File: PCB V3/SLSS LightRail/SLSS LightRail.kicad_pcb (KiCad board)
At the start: 2 copper layers, 18.1 x 32.8 mm, 1 part

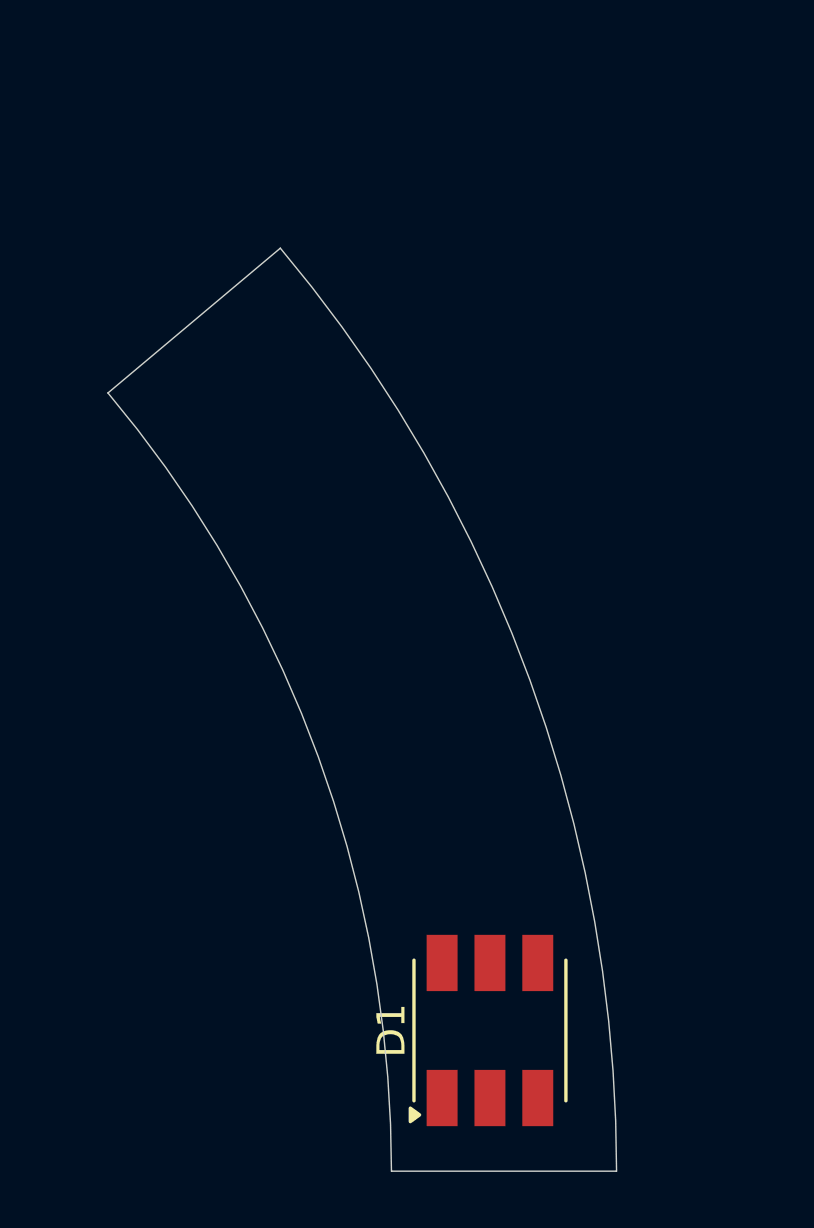
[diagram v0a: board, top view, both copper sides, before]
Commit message: light rail PCB
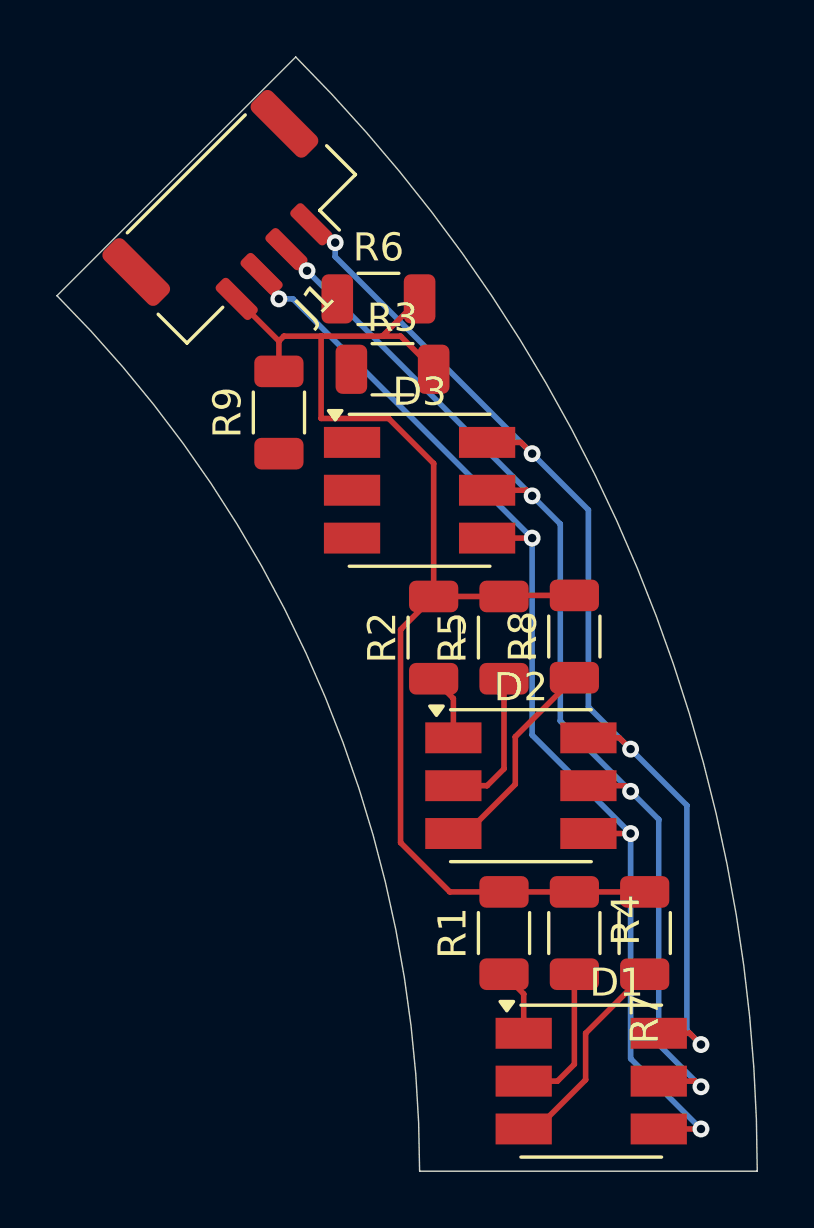
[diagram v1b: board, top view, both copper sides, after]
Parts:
- added D2: LED_RGB, LED_SMD:LED_RGB_5050-6, F.Cu at (197.6, 86.3)
- added D3: LED_RGB, LED_SMD:LED_RGB_5050-6, F.Cu at (194.0, 75.8)
- added J1: Conn_01x04, Connector_JST:JST_GH_SM04B-GHS-TB_1x04-1MP_P1.25mm_Horizontal, F.Cu at (187.5, 66.4)
- added R1: 51R, Resistor_SMD:R_1206_3216Metric, F.Cu at (197.0, 91.5)
- added R2: 51R, Resistor_SMD:R_1206_3216Metric, F.Cu at (194.5, 81.0)
- added R3: 51R, Resistor_SMD:R_1206_3216Metric, F.Cu at (193.0, 71.5)
- added R4: 62R, Resistor_SMD:R_1206_3216Metric, F.Cu at (199.5, 91.5)
- added R5: 62R, Resistor_SMD:R_1206_3216Metric, F.Cu at (197.0, 81.0)
- added R6: 62R, Resistor_SMD:R_1206_3216Metric, F.Cu at (192.5, 69.0)
- added R7: 51R, Resistor_SMD:R_1206_3216Metric, F.Cu at (202.0, 91.5)
- added R8: 51R, Resistor_SMD:R_1206_3216Metric, F.Cu at (199.5, 81.0)
- added R9: 51R, Resistor_SMD:R_1206_3216Metric, F.Cu at (189.0, 73.0)
- moved D1 4.02 mm to (200.1, 96.8), turned to 0 degrees
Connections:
- D1 pad 1: unconnected-(D1-RK-Pad1) -> Net-(D1-RK)
- D1 pad 2: unconnected-(D1-GK-Pad2) -> Net-(D1-GK)
- D1 pad 3: unconnected-(D1-BK-Pad3) -> Net-(D1-BK)
- D1 pad 4: unconnected-(D1-BA-Pad4) -> Net-(D1-BA)
- D1 pad 5: unconnected-(D1-GA-Pad5) -> Net-(D1-GA)
- D1 pad 6: unconnected-(D1-RA-Pad6) -> Net-(D1-RA)
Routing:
- net Net-(J1-Pin_4): track 0.00 -> 47.2 mm
- net Net-(D1-BA): track 0.00 -> 41.7 mm, vias 0 -> 4
- net Net-(D1-GA): track 0.00 -> 41.0 mm, vias 0 -> 4
- net Net-(D1-RA): track 0.00 -> 39.9 mm, vias 0 -> 4
- net Net-(D2-BK): track 0.00 -> 7.58 mm
- net Net-(D1-BK): track 0.00 -> 7.55 mm
- net Net-(D2-GK): track 0.00 -> 5.25 mm
- net Net-(D1-GK): track 0.00 -> 5.25 mm
- net Net-(D2-RK): track 0.00 -> 2.39 mm
- net Net-(D1-RK): track 0.00 -> 2.39 mm
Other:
- board size 18.1 x 32.8 mm -> 24.9 x 39.6 mm
- board text added: "${REFERENCE}"

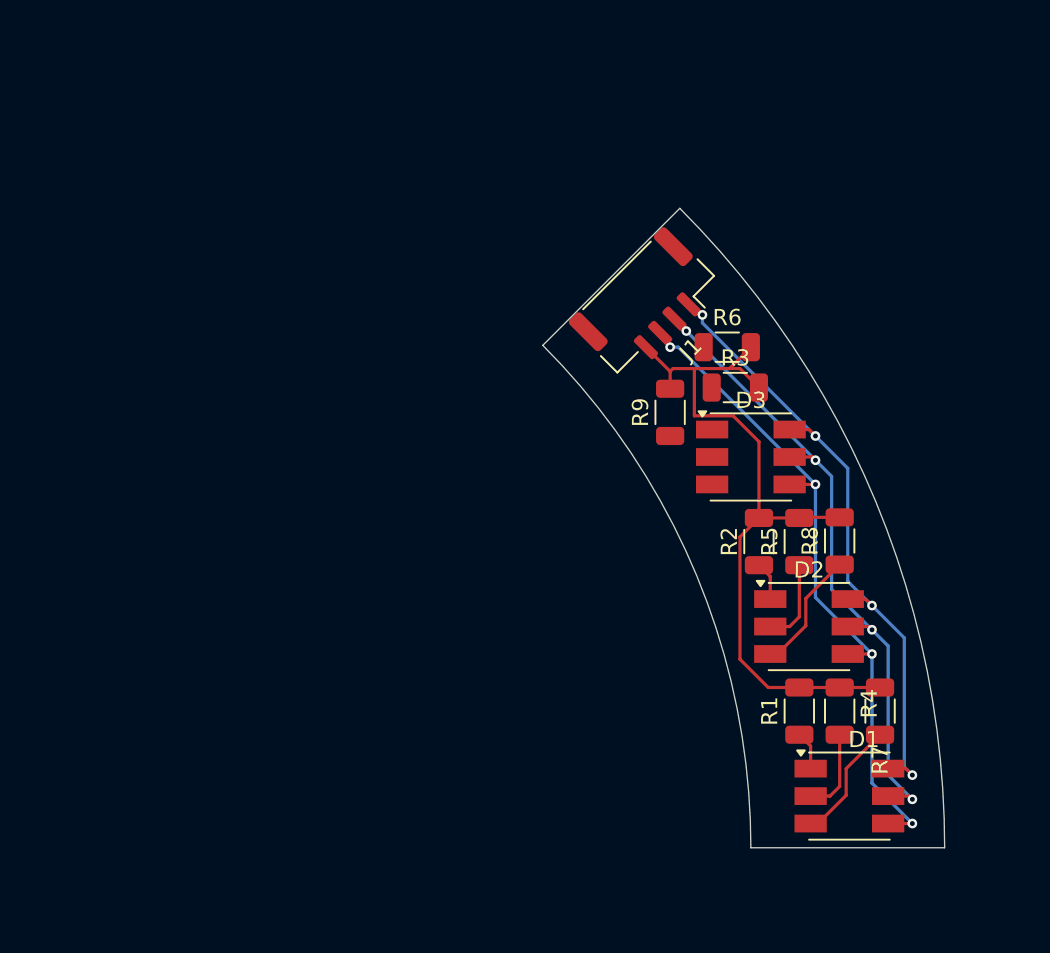
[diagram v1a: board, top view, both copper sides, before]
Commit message: Finished Lightrail PCB
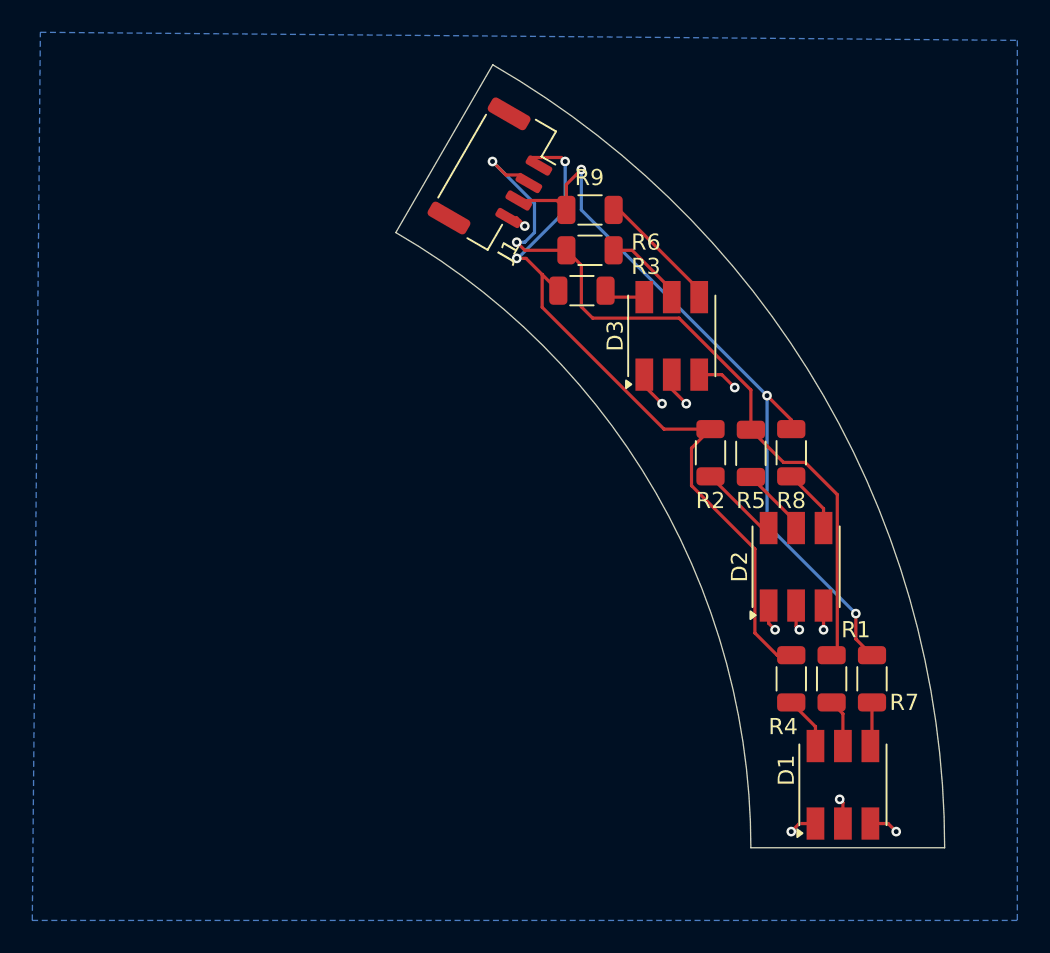
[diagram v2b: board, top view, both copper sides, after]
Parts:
- moved R9 13.5 mm to (184.0, 60.5), turned to 0 degrees
- moved J1 12.1 mm to (178.3, 58.5), turned to -120 degrees
- moved R3 11.2 mm to (183.5, 65.5)
- moved R6 10.4 mm to (184.0, 63.0)
- moved D3 8.96 mm to (189.1, 68.3), turned to 90 degrees
- moved R2 6.26 mm to (191.5, 75.5), turned to -90 degrees
- moved R8 6.23 mm to (196.5, 75.5), turned to -90 degrees
- moved R5 6.23 mm to (194.0, 75.6), turned to -90 degrees
- moved D2 3.79 mm to (196.8, 82.6), turned to 90 degrees
- moved R1 2.06 mm to (196.5, 89.5), turned to -90 degrees
- moved R4 2.06 mm to (199.0, 89.5), turned to 90 degrees
- moved R7 2.06 mm to (201.5, 89.5), turned to -90 degrees
- moved D1 0.81 mm to (199.7, 96.1), turned to 90 degrees
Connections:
- D1 pad 1: Net-(D1-RK) -> Net-(D1-BK)
- D1 pad 2: Net-(D1-GK) -> Net-(D1-BK)
- D2 pad 1: Net-(D2-RK) -> Net-(D1-BK)
- D2 pad 2: Net-(D2-GK) -> Net-(D1-BK)
- D2 pad 3: Net-(D2-BK) -> Net-(D1-BK)
- D2 pad 4: Net-(D1-BA) -> Net-(D2-BA)
- D2 pad 5: Net-(D1-GA) -> Net-(D2-GA)
- D2 pad 6: Net-(D1-RA) -> Net-(D2-RA)
- D3 pad 1: Net-(D3-RK) -> Net-(D1-BK)
- D3 pad 2: Net-(D3-GK) -> Net-(D1-BK)
- D3 pad 3: Net-(D3-BK) -> Net-(D1-BK)
- D3 pad 4: Net-(D1-BA) -> Net-(D3-BA)
- D3 pad 5: Net-(D1-GA) -> Net-(D3-GA)
- D3 pad 6: Net-(D1-RA) -> Net-(D3-RA)
- J1 pad 1: Net-(D1-RA) -> Net-(J1-Pin_1)
- J1 pad 2: Net-(D1-GA) -> Net-(J1-Pin_2)
- J1 pad 3: Net-(D1-BA) -> Net-(J1-Pin_3)
- J1 pad 4: Net-(J1-Pin_4) -> Net-(D1-BK)
- R1 pad 1: Net-(D1-RK) -> Net-(J1-Pin_1)
- R1 pad 2: Net-(J1-Pin_4) -> Net-(D1-RA)
- R2 pad 1: Net-(D2-RK) -> Net-(J1-Pin_1)
- R2 pad 2: Net-(J1-Pin_4) -> Net-(D2-RA)
- R3 pad 1: Net-(D3-RK) -> Net-(J1-Pin_1)
- R3 pad 2: Net-(J1-Pin_4) -> Net-(D3-RA)
- R4 pad 1: Net-(J1-Pin_4) -> Net-(D1-GA)
- R4 pad 2: Net-(D1-GK) -> Net-(J1-Pin_2)
- R5 pad 1: Net-(D2-GK) -> Net-(J1-Pin_2)
- R5 pad 2: Net-(J1-Pin_4) -> Net-(D2-GA)
- R6 pad 1: Net-(D3-GK) -> Net-(J1-Pin_2)
- R6 pad 2: Net-(J1-Pin_4) -> Net-(D3-GA)
- R7 pad 1: Net-(D1-BK) -> Net-(J1-Pin_3)
- R7 pad 2: Net-(J1-Pin_4) -> Net-(D1-BA)
- R8 pad 1: Net-(D2-BK) -> Net-(J1-Pin_3)
- R8 pad 2: Net-(J1-Pin_4) -> Net-(D2-BA)
- R9 pad 1: Net-(D3-BK) -> Net-(J1-Pin_3)
- R9 pad 2: Net-(J1-Pin_4) -> Net-(D3-BA)
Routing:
- net Net-(J1-Pin_2): track 0.00 -> 48.3 mm, vias 0 -> 2
- net Net-(J1-Pin_4): track 47.2 -> 0.00 mm
- net Net-(J1-Pin_3): track 0.00 -> 46.3 mm, vias 0 -> 3
- net Net-(J1-Pin_1): track 0.00 -> 46.0 mm, vias 0 -> 2
- net Net-(D1-BA): track 41.7 -> 2.74 mm, vias 4 -> 0
- net Net-(D1-GA): track 41.0 -> 2.99 mm, vias 4 -> 0
- net Net-(D1-RA): track 39.9 -> 3.32 mm, vias 4 -> 0
- net Net-(D1-BK): track 7.55 -> 18.0 mm, vias 0 -> 10
- net Net-(D3-BA): track 0.00 -> 7.80 mm
- net Net-(D2-BK): track 7.58 -> 0.00 mm
- net Net-(D2-GK): track 5.25 -> 0.00 mm
- net Net-(D1-GK): track 5.25 -> 0.00 mm
- net Net-(D3-GA): track 0.00 -> 5.06 mm
- net Net-(D2-RA): track 0.00 -> 4.93 mm
- net Net-(D2-GA): track 0.00 -> 4.32 mm
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- added copper zone on B.Cu, net Net-(D1-BK)
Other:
- board size 24.9 x 39.6 mm -> 34 x 48.5 mm
- board text removed: "${REFERENCE}"

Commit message: PCB size fix
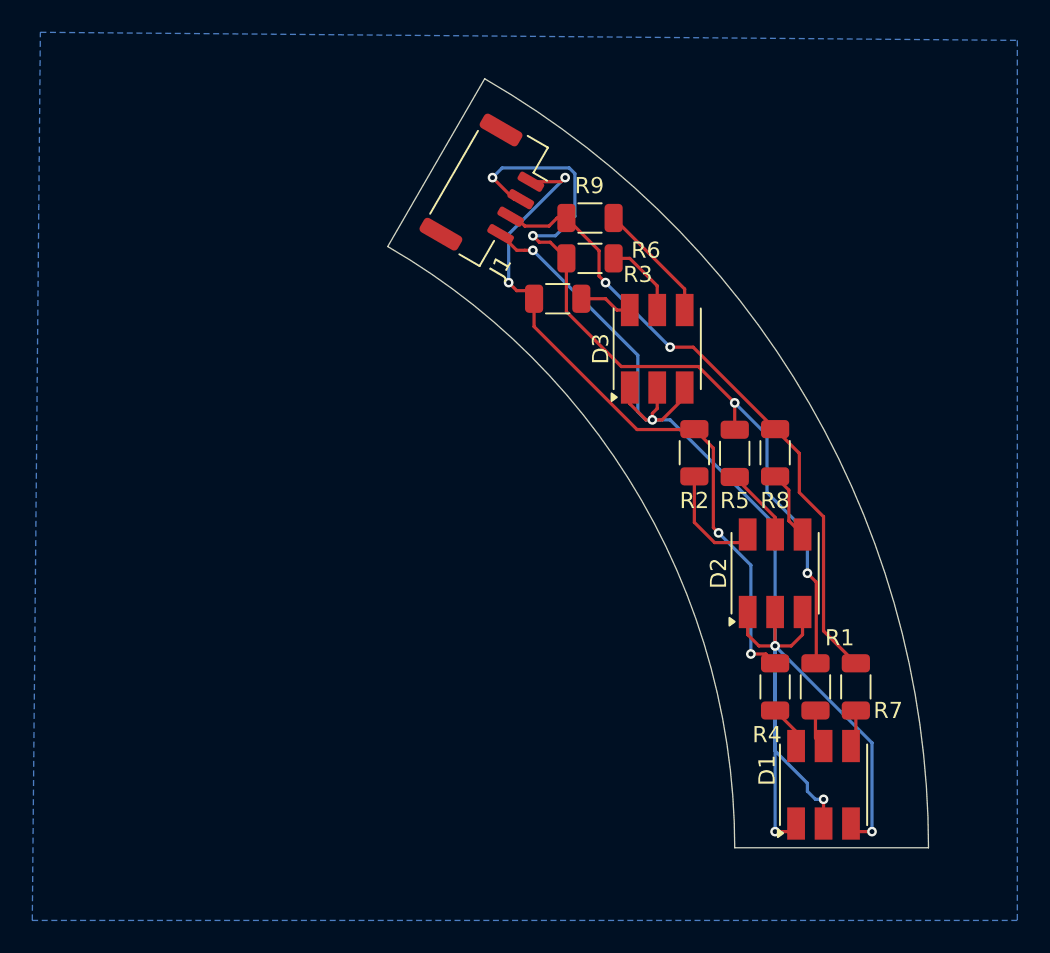
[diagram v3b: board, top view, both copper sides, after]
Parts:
- moved R3 1.58 mm to (182.0, 66.0)
- moved D2 1.36 mm to (195.5, 83.0)
- moved D3 1.20 mm to (188.2, 69.1)
- moved D1 1.20 mm to (198.5, 96.1)
- moved J1 1.12 mm to (177.8, 59.5)
- moved R1 1.12 mm to (195.5, 90.0)
- moved R4 1.12 mm to (198.0, 90.0)
- moved R7 1.12 mm to (200.5, 90.0)
- moved R2 1.00 mm to (190.5, 75.5)
- moved R5 1.00 mm to (193.0, 75.6)
- moved R8 1.00 mm to (195.5, 75.5)
- moved R6 0.50 mm to (184.0, 63.5)
- moved R9 0.50 mm to (184.0, 61.0)
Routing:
- net Net-(D1-BK): track 18.0 -> 92.3 mm, vias 10 -> 6
- net Net-(J1-Pin_3): track 46.3 -> 39.7 mm, vias 3 -> 2
- net Net-(J1-Pin_2): track 48.3 -> 52.2 mm, vias 2 -> 4
- net Net-(J1-Pin_1): track 46.0 -> 43.6 mm, vias 2 -> 4
- net Net-(D2-RA): track 4.93 -> 6.88 mm
- net Net-(D3-RA): track 2.00 -> 3.29 mm
- net Net-(D1-RA): track 3.32 -> 2.74 mm
- net Net-(D1-GA): track 2.99 -> 2.41 mm
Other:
- board size 34 x 48.5 mm -> 33.5 x 47.6 mm
